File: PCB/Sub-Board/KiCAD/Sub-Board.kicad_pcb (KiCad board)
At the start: 4 copper layers, 50.5 x 113 mm, 200 parts, among them J1 Conn_02x08, J10 Type, J11 Power/I2C, J12 Address, J13 Power/I2C, J14 Address, J15 GPIO, J16 Type, J17 GPIO, J18 Type, J19 Power/I2C, J2 Conn_01x04_Pin, J20 Address, J21 Power/I2C, J22 Address, J23 GPIO, J24 Type, J25 GPIO, J26 Type, J27 Power/I2C, J28 Address, J29 Power/I2C, J3 Power/I2C, J30 Address, J31 GPIO, J32 Type, J33 GPIO, J34 Type, J4 Address, J5 Power/I2C, J6 Address, J7 GPIO, J8 Type, J9 GPIO, SW1 SW_DIP_x07, U1 TPS629210DRLR, U2 74HC165, U3 STM32F401VETx, U4 74HC165, U5 74HC165, U6 74HC165, U7 74HC165, Y1 26 MHz

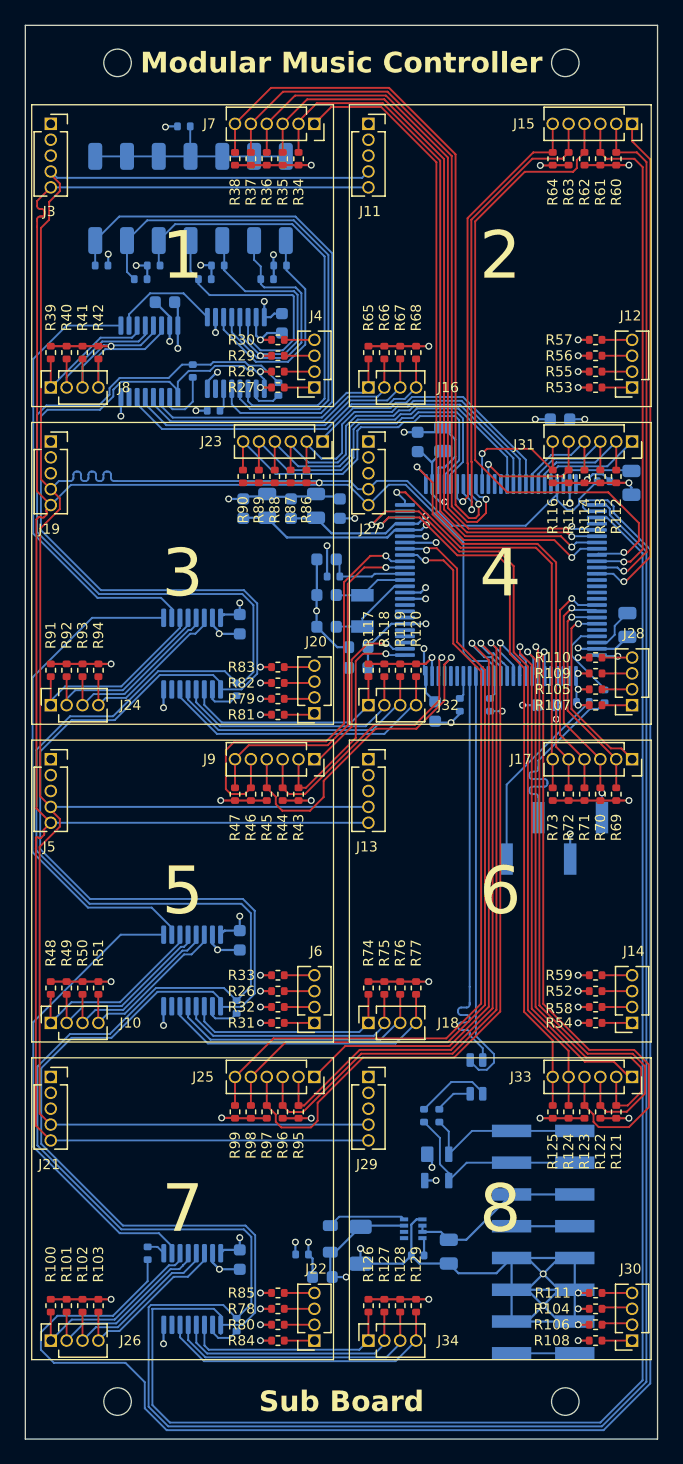
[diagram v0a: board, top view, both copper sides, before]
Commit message: PCB Sub Board: Revision 2
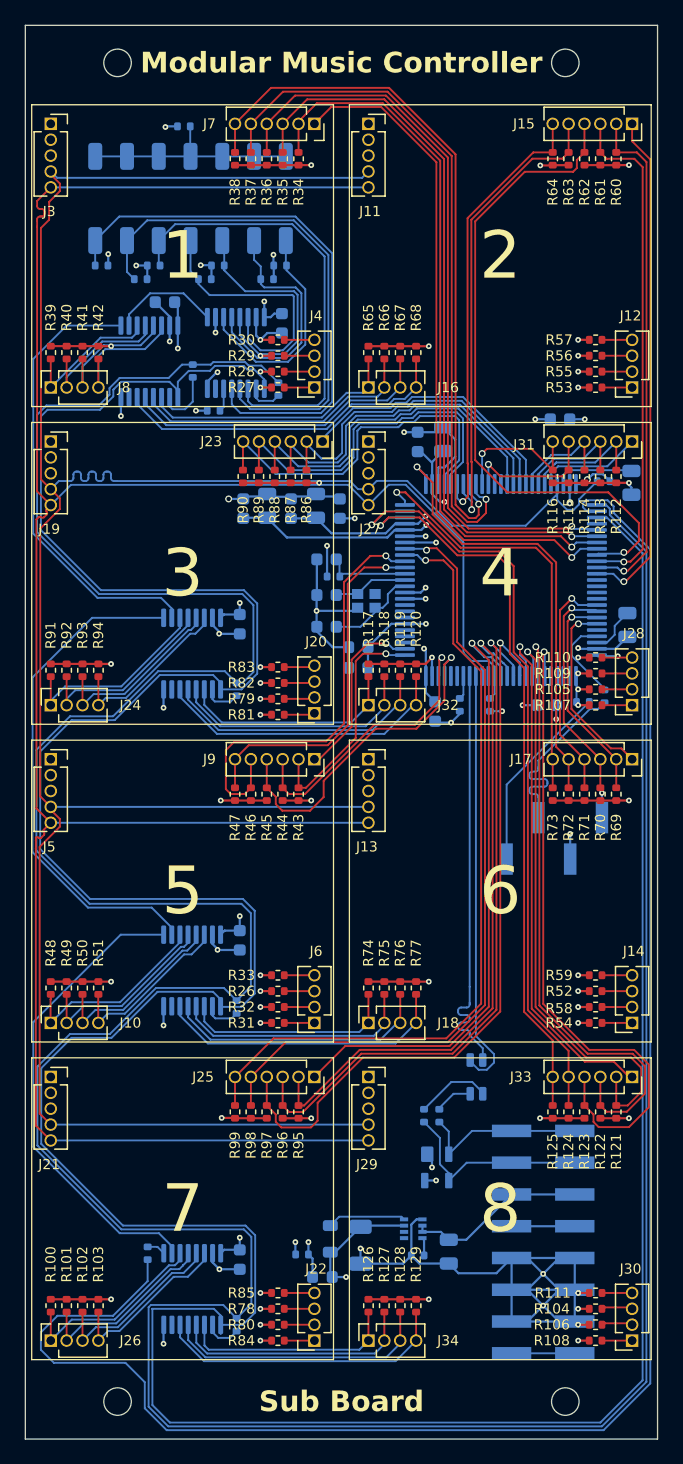
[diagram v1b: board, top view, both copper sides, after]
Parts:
- FB1: value 600Ω @ 100MHz ~300-500mA -> Laird HZ0603C651R-10
- J1: value Conn_02x08 -> Harwin M20-8760846
- J10, J16, J18, J24, J26, J32, J34, J8: value Type -> Samtec RSM-104-02-L-S
- J11, J13, J19, J21, J27, J29, J3, J5: value Power/I2C -> Samtec RSM-105-02-L-S
- J12, J14, J20, J22, J28, J30, J4, J6: value Address -> Samtec RSM-104-02-L-S
- J15, J17, J23, J25, J31, J33, J7, J9: value GPIO -> Samtec RSM-106-02-L-S
- J2: value Conn_01x04_Pin -> Harwin M20-8770446
- L1: value Choke_Wurth_WE-CNSW_744232090 -> Wuerth 744232090
- SW1: value SW_DIP_x07 -> CTS 219-7LPSTR
- U2, U4, U5, U6, U7: value 74HC165 -> Nexperia 74HC165PW,118
- U3: value STM32F401VETx -> STM32F401VET6
- Y1: value 26 MHz -> Kyocera CX2016DB26000H0FLJC2; footprint Crystal:Crystal_SMD_3215-2Pin_3.2x1.5mm -> CX2016DB26000H0FLJC2:OSC_CX2016DB26000H0FLJC2
- moved Y1 0.86 mm to (129.0, 84.1)
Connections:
- Y1 pad 1: /STM32-MCU/PH1 -> /STM32-MCU/PH0
- Y1 pad 2: /STM32-MCU/PH0 -> GND
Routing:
- net GND: track 249.6 -> 253.2 mm
